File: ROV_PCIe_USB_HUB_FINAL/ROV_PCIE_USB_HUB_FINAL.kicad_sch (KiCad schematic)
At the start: 17 parts, among them J1 SFV16R-1STBE1HLF, J2 1053131102, J3 1053071202, Q1 DMP3018SFV

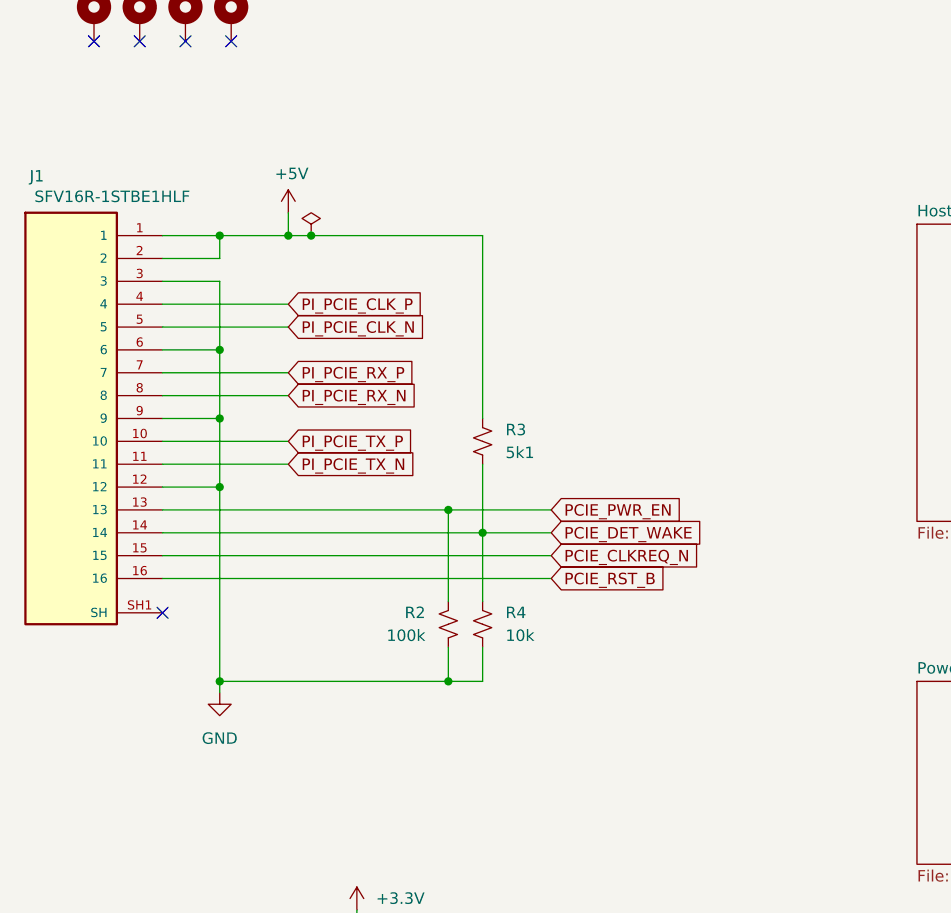
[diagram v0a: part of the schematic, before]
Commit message: changes
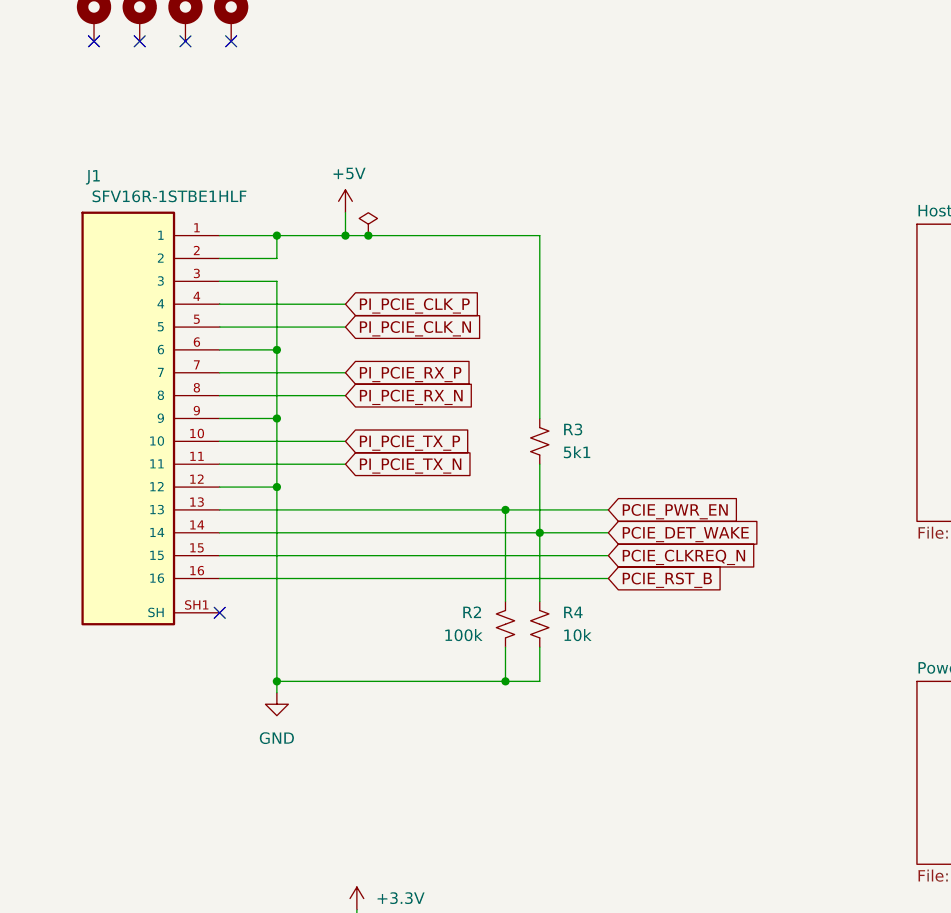
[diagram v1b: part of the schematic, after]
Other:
- moved on the sheet: J1, R2, R3, R4
